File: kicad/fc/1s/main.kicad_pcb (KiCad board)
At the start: 2 copper layers, 40.2 x 46.1 mm, 34 parts, among them J1 Conn_01x14, J10 Conn_01x01_Pin, J11 Conn_01x01_Pin, J12 Conn_01x01_Pin, J13 Conn_01x01_Pin, J14 Conn_01x01_Pin, J15 Conn_01x03_Socket, J16 Conn_01x03_Socket, J17 Conn_01x01_Pin, J18 Conn_01x01_Pin, J19 Conn_01x01_Pin, J2 Conn_01x14_Socket, J20 Conn_01x01_Pin, J21 Conn_01x01_Pin, J22 Conn_01x01_Pin, J23 Conn_01x03_Socket, J24 Conn_01x03_Socket, J25 Conn_01x01_Pin, J26 Conn_01x01_Pin, J27 Conn_02x04_Odd_Even, J3 Conn_01x01_Pin, J4 Conn_01x03_Socket, J5 Conn_01x01_Pin, J7 Conn_01x01_Pin, J8 Conn_01x01_Pin, J9 Conn_01x01_Pin

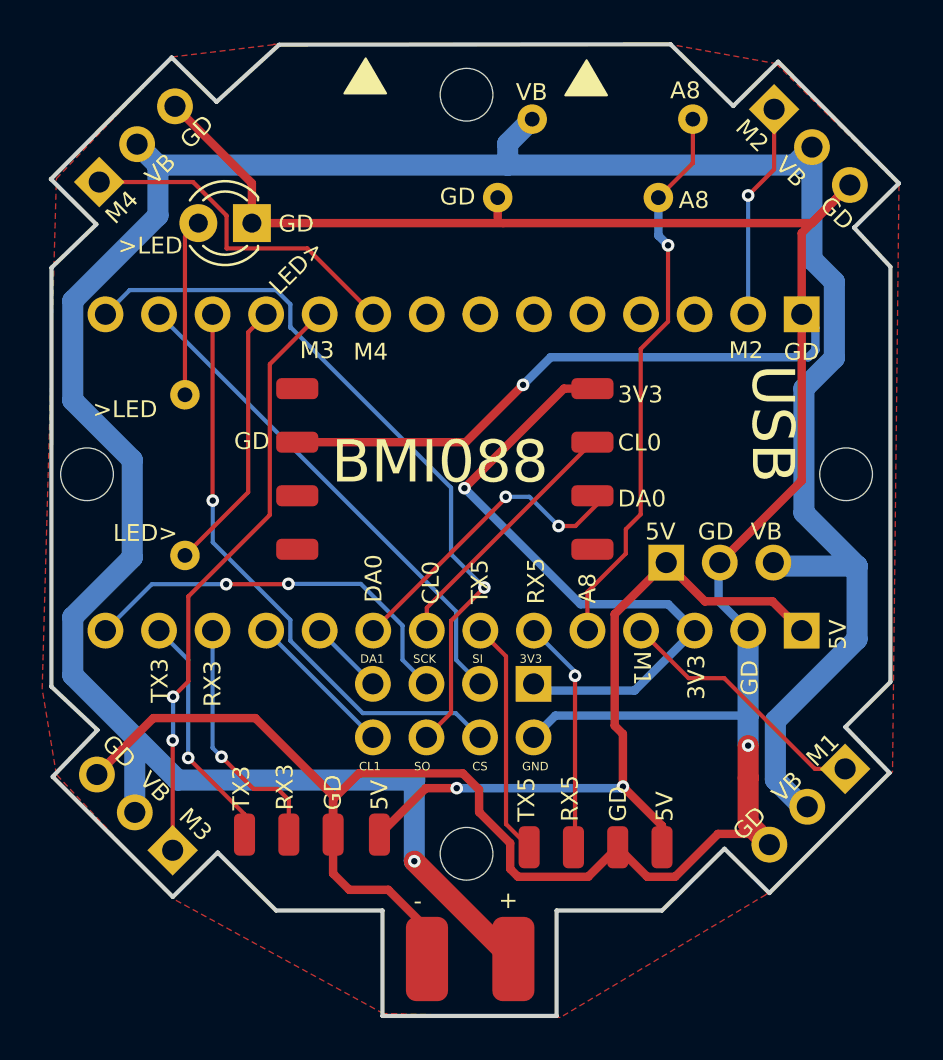
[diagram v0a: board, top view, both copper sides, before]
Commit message: modified:   kicad/fc/1s/main.kicad_pcb
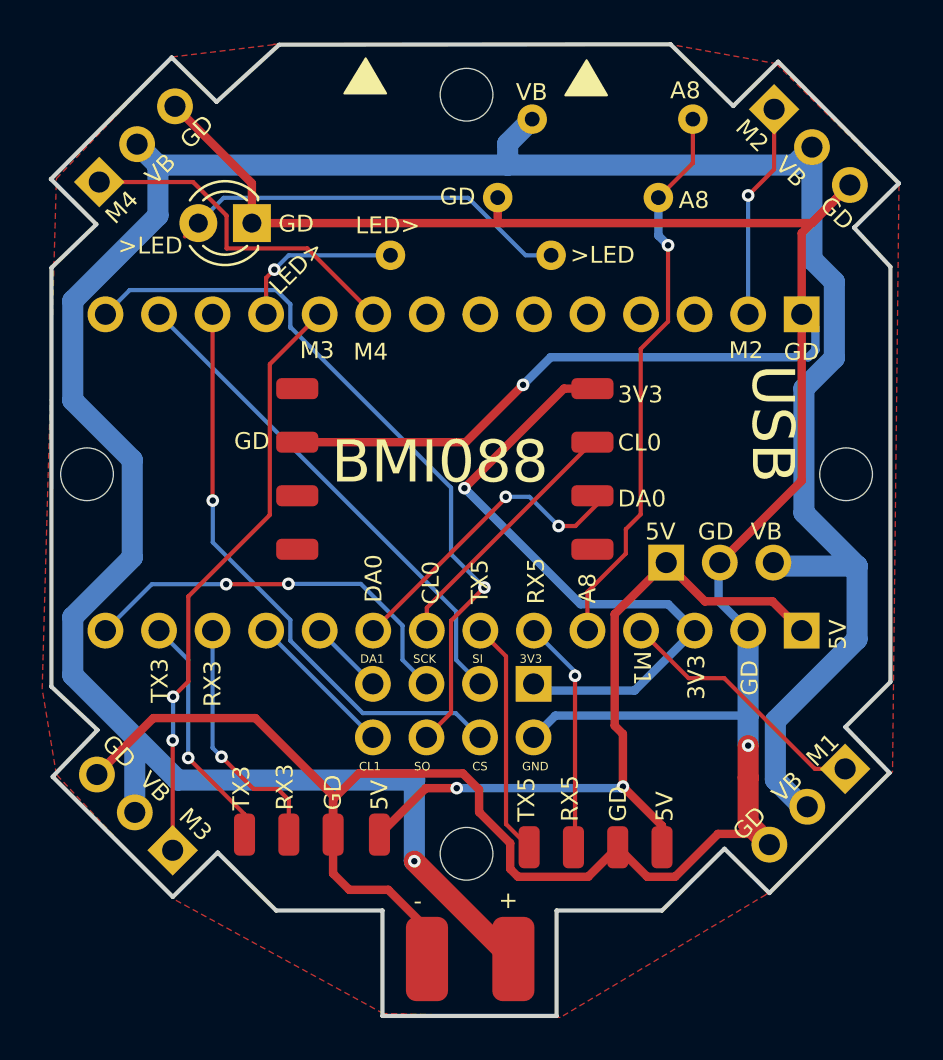
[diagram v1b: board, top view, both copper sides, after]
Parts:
- moved R1 17.9 mm to (148.8, 74.9), turned to 180 degrees
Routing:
- net Net-(D1-A): track 8.40 -> 19.3 mm
- net /LED: track 13.0 -> 8.07 mm, vias 0 -> 1
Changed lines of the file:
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@@
 	(footprint "Resistor_THT:R_Axial_DIN0204_L3.6mm_D1.6mm_P7.62mm_Horizontal"
 		(layer "F.Cu")
-		(at 132.675 82.79 -90)
+		(at 148.791324 74.924901 180)
 		(descr "Resistor, Axial_DIN0204 series, Axial, Horizontal, pin pitch=7.62mm, 0.167W, length*diameter=3.6*1.6mm^2, http://cdn-reichelt.de/documents/datenblatt/B400/1_4W%23YAG.pdf")
 		(tags "Resistor Axial_DIN0204 series Axial Horizontal pin pitch 7.62mm 0.167W length 3.6mm diameter 1.6mm")
 		(property "Reference" "R1"
-			(at 3.81 0 90)
+			(at 3.81 0 0)
 			(layer "F.SilkS")
 			(hide yes)
@@
 		)
 		(property "Value" "R_LED"
-			(at 3.81 1.92 90)
+			(at 3.81 1.92 0)
 			(layer "F.Fab")
 			(hide yes)
@@
 		)
 		(property "Datasheet" ""
-			(at 0 0 90)
+			(at 0 0 0)
 			(layer "F.Fab")
 			(hide yes)
@@
 		)
 		(property "Description" "Resistor"
-			(at 0 0 90)
+			(at 0 0 0)
 			(layer "F.Fab")
 			(hide yes)
@@
 		(duplicate_pad_numbers_are_jumpers no)
 		(pad "1" thru_hole circle
-			(at -1.25 0 270)
+			(at -1.25 0 180)
 			(size 1.4 1.4)
 			(drill 0.7)
@@
 		)
 		(pad "2" thru_hole circle
-			(at 6.37 0 270)
+			(at 6.37 0 180)
 			(size 1.4 1.4)
 			(drill 0.7)
@@
 	)
 	(gr_text ">LED"
-		(at 128.3 82.7 0)
-		(layer "F.SilkS")
-		(effects
-			(font
-				(size 0.8 0.8)
-				(thickness 0.15)
-			)
-			(justify left bottom)
-		)
-	)
-	(gr_text "LED>"
-		(at 129.26 88.57 0)
+		(at 129.499815 74.938153 0)
 		(layer "F.SilkS")
 		(effects
@@
 		)
 	)
-	(gr_text ">LED"
-		(at 129.499815 74.938153 0)
+	(gr_text "GD"
+		(at 135 84.21 0)
 		(layer "F.SilkS")
 		(effects
@@
 	)
 	(gr_text "GD"
-		(at 135 84.21 0)
+		(at 137.1 73.9 0)
 		(layer "F.SilkS")
 		(effects
@@
 		)
 	)
-	(gr_text "GD"
-		(at 137.1 73.9 0)
+	(gr_text "M3"
+		(at 138.119148 79.9 0)
 		(layer "F.SilkS")
 		(effects
@@
 		)
 	)
-	(gr_text "M3"
-		(at 138.119148 79.9 0)
+	(gr_text "M4"
+		(at 140.663107 79.971888 0)
 		(layer "F.SilkS")
 		(effects
@@
 		)
 	)
-	(gr_text "M4"
-		(at 140.663107 79.971888 0)
+	(gr_text "LED>"
+		(at 140.755653 73.980584 0)
 		(layer "F.SilkS")
 		(effects
@@
 		)
 	)
+	(gr_text ">LED"
+		(at 150.943372 75.378899 0)
+		(layer "F.SilkS")
+		(effects
+			(font
+				(size 0.8 0.8)
+				(thickness 0.15)
+			)
+			(justify left bottom)
+		)
+	)
 	(gr_text "3V3"
 		(at 153.2 82 0)
@@
 		)
 	)
+	(gr_text "R 100Ω"
+		(at 148.609151 75.511735 0)
+		(layer "B.SilkS")
+		(effects
+			(font
+				(size 0.8 0.8)
+				(thickness 0.15)
+			)
+			(justify left bottom mirror)
+		)
+	)
 	(gr_text "5V"
 		(at 156 88.5 0)
@@
 		)
 	)
-	(gr_text "R 100Ω"
-		(at 133.15 82.95 90)
-		(layer "B.SilkS")
-		(effects
-			(font
-				(size 0.8 0.8)
-				(thickness 0.15)
-			)
-			(justify left bottom mirror)
-		)
-	)
 	(gr_text "CS"
 		(at 134.51 78.9 90)
@@
 	)
 	(segment
+		(start 144.145 91.645)
+		(end 152 83.79)
+		(width 0.2)
+		(layer "F.Cu")
+		(net "/SCL0")
+	)
+	(segment
+		(start 144.145 92.725)
+		(end 144.145 91.645)
+		(width 0.2)
+		(layer "F.Cu")
+		(net "/SCL0")
+	)
+	(segment
+		(start 131.445 77.725)
+		(end 145.535 91.815)
+		(width 0.2)
+		(layer "B.Cu")
+		(net "/MOSI")
+	)
+	(segment
+		(start 145.535 91.815)
+		(end 145.535 94.115961)
+		(width 0.2)
+		(layer "B.Cu")
+		(net "/MOSI")
+	)
+	(segment
+		(start 145.535 94.115961)
+		(end 146.668695 95.249656)
+		(width 0.2)
+		(layer "B.Cu")
+		(net "/MOSI")
+	)
+	(segment
 		(start 133.993688 86.558557)
 		(end 134.057247 86.622117)
@@
 	)
 	(segment
-		(start 131.445 77.725)
-		(end 145.535 91.815)
+		(start 134.630131 90.523599)
+		(end 137.565258 90.523599)
+		(width 0.2)
+		(layer "F.Cu")
+		(net "/SCK")
+	)
+	(segment
+		(start 137.565258 90.523599)
+		(end 137.580262 90.508595)
+		(width 0.2)
+		(layer "F.Cu")
+		(net "/SCK")
+	)
+	(via
+		(at 134.630131 90.523599)
+		(size 0.6)
+		(drill 0.3)
+		(layers "F.Cu" "B.Cu")
+		(net "/SCK")
+	)
+	(via
+		(at 137.580262 90.508595)
+		(size 0.6)
+		(drill 0.3)
+		(layers "F.Cu" "B.Cu")
+		(net "/SCK")
+	)
+	(segment
+		(start 141.014941 90.508595)
+		(end 137.580262 90.508595)
 		(width 0.2)
 		(layer "B.Cu")
-		(net "/MOSI")
+		(net "/SCK")
 	)
 	(segment
-		(start 145.535 91.815)
-		(end 145.535 94.115961)
+		(start 134.630131 90.523599)
+		(end 134.669611 90.523599)
 		(width 0.2)
 		(layer "B.Cu")
-		(net "/MOSI")
+		(net "/SCK")
 	)
 	(segment
-		(start 145.535 94.115961)
-		(end 146.668695 95.249656)
+		(start 131.106401 90.523599)
+		(end 134.630131 90.523599)
 		(width 0.2)
 		(layer "B.Cu")
-		(net "/MOSI")
+		(net "/SCK")
+	)
+	(segment
+		(start 142.995 92.488654)
+		(end 141.014941 90.508595)
+		(width 0.2)
+		(layer "B.Cu")
+		(net "/SCK")
+	)
+	(segment
+		(start 128.905 92.725)
+		(end 131.106401 90.523599)
+		(width 0.2)
+		(layer "B.Cu")
+		(net "/SCK")
+	)
+	(segment
+		(start 142.995 94.115961)
+		(end 142.995 92.488654)
+		(width 0.2)
+		(layer "B.Cu")
+		(net "/SCK")
+	)
+	(segment
+		(start 144.128695 95.249656)
+		(end 142.995 94.115961)
+		(width 0.2)
+		(layer "B.Cu")
+		(net "/SCK")
 	)
 	(segment
@@
 	)
 	(segment
-		(start 134.630131 90.523599)
-		(end 137.565258 90.523599)
-		(width 0.2)
-		(layer "F.Cu")
-		(net "/SCK")
-	)
-	(segment
-		(start 137.565258 90.523599)
-		(end 137.580262 90.508595)
+		(start 141.588695 95.248695)
+		(end 141.588695 95.249656)
 		(width 0.2)
 		(layer "F.Cu")
-		(net "/SCK")
-	)
-	(via
-		(at 134.630131 90.523599)
-		(size 0.6)
-		(drill 0.3)
-		(layers "F.Cu" "B.Cu")
-		(net "/SCK")
-	)
-	(via
-		(at 137.580262 90.508595)
-		(size 0.6)
-		(drill 0.3)
-		(layers "F.Cu" "B.Cu")
-		(net "/SCK")
-	)
-	(segment
-		(start 141.014941 90.508595)
-		(end 137.580262 90.508595)
-		(width 0.2)
-		(layer "B.Cu")
-		(net "/SCK")
-	)
-	(segment
-		(start 134.630131 90.523599)
-		(end 134.669611 90.523599)
-		(width 0.2)
-		(layer "B.Cu")
-		(net "/SCK")
-	)
-	(segment
-		(start 131.106401 90.523599)
-		(end 134.630131 90.523599)
-		(width 0.2)
-		(layer "B.Cu")
-		(net "/SCK")
-	)
-	(segment
-		(start 142.995 92.488654)
-		(end 141.014941 90.508595)
-		(width 0.2)
-		(layer "B.Cu")
-		(net "/SCK")
-	)
-	(segment
-		(start 128.905 92.725)
-		(end 131.106401 90.523599)
-		(width 0.2)
-		(layer "B.Cu")
-		(net "/SCK")
-	)
-	(segment
-		(start 142.995 94.115961)
-		(end 142.995 92.488654)
-		(width 0.2)
-		(layer "B.Cu")
-		(net "/SCK")
+		(net "/SDA1")
 	)
 	(segment
-		(start 144.128695 95.249656)
-		(end 142.995 94.115961)
+		(start 139.065 92.725)
+		(end 141.588695 95.248695)
 		(width 0.2)
 		(layer "B.Cu")
-		(net "/SCK")
+		(net "/SDA1")
 	)
 	(segment
@@
 	)
 	(segment
-		(start 141.588695 95.248695)
-		(end 141.588695 95.249656)
-		(width 0.2)
-		(layer "F.Cu")
-		(net "/SDA1")
-	)
-	(segment
-		(start 139.065 92.725)
-		(end 141.588695 95.248695)
-		(width 0.2)
-		(layer "B.Cu")
-		(net "/SDA1")
-	)
-	(segment
-		(start 144.145 91.645)
-		(end 152 83.79)
-		(width 0.2)
-		(layer "F.Cu")
-		(net "/SCL0")
-	)
-	(segment
-		(start 144.145 92.725)
-		(end 144.145 91.645)
-		(width 0.2)
-		(layer "F.Cu")
-		(net "/SCL0")
-	)
-	(segment
 		(start 147.902579 93.942579)
 		(end 147.902579 101.902579)
@@
 	)
 	(segment
-		(start 132.675 74.035)
-		(end 132.675 81.54)
+		(start 146.103439 72.2)
+		(end 148.82834 74.924901)
 		(width 0.2)
-		(layer "F.Cu")
+		(layer "B.Cu")
+		(net "Net-(D1-A)")
+	)
+	(segment
+		(start 148.82834 74.924901)
+		(end 150.041324 74.924901)
+		(width 0.2)
+		(layer "B.Cu")
+		(net "Net-(D1-A)")
+	)
+	(segment
+		(start 134.51 72.2)
+		(end 146.103439 72.2)
+		(width 0.2)
+		(layer "B.Cu")
+		(net "Net-(D1-A)")
+	)
+	(segment
+		(start 133.31 73.4)
+		(end 134.51 72.2)
+		(width 0.2)
+		(layer "B.Cu")
 		(net "Net-(D1-A)")
 	)
@@
 	(segment
 		(start 136.525 77.725)
-		(end 135.675 78.575)
+		(end 136.525 75.996062)
 		(width 0.2)
 		(layer "F.Cu")
@@
 	)
 	(segment
-		(start 135.675 86.16)
-		(end 132.675 89.16)
+		(start 136.525 75.996062)
+		(end 136.914829 75.606233)
 		(width 0.2)
 		(layer "F.Cu")
 		(net "/LED")
 	)
+	(via
+		(at 136.914829 75.606233)
+		(size 0.6)
+		(drill 0.3)
+		(layers "F.Cu" "B.Cu")
+		(net "/LED")
+	)
 	(segment
-		(start 135.675 78.575)
-		(end 135.675 86.16)
+		(start 136.914829 75.606233)
+		(end 137.596161 74.924901)
 		(width 0.2)
-		(layer "F.Cu")
+		(layer "B.Cu")
+		(net "/LED")
+	)
+	(segment
+		(start 137.596161 74.924901)
+		(end 142.421324 74.924901)
+		(width 0.2)
+		(layer "B.Cu")
 		(net "/LED")
 	)
